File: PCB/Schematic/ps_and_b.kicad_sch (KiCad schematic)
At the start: 23 parts, among them J1 CQ-USB-C16PSMT01, J3 JST_02, SW5 SW_Nidec_CAS-120A1, U1 AMS1117-3.3, U3 CH343P, U4 CN3063-SOIC8, U9 TPS61023DRLR

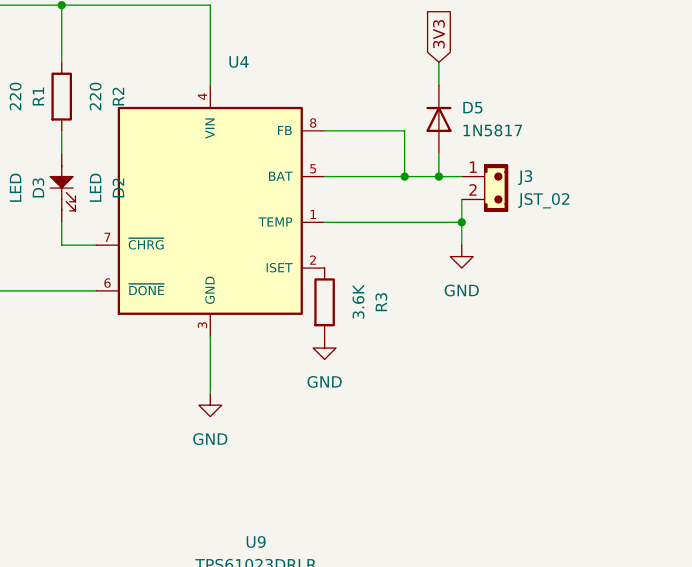
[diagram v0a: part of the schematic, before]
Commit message: Add files via upload
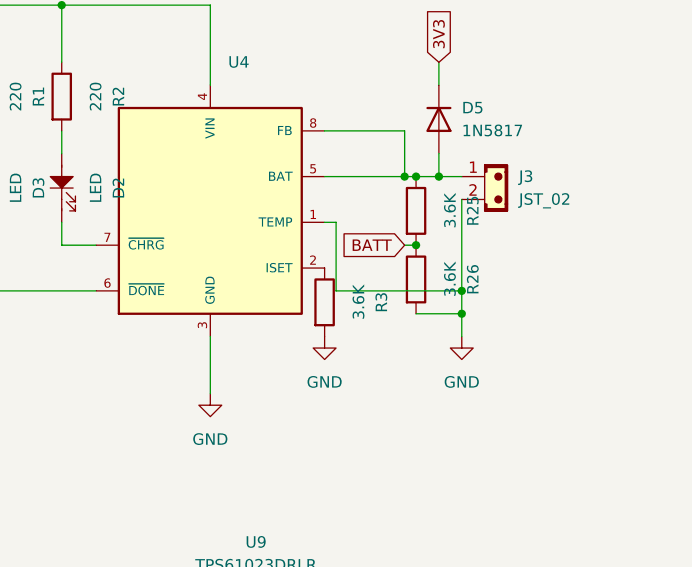
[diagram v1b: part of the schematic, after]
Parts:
- added R25, R26: 3.6K, Resistor_SMD:R_0805_2012Metric, symbol Device:R
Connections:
- net GND: now also R26.2
- net at D5.2 (A), J3.1, U4.5 (BAT)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: now also R25.1
- new net BATT: R25.2, R26.1
